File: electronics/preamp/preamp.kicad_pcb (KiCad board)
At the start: 2 copper layers, 24.8 x 24.8 mm, 33 parts, among them J1 Conn_01x01, J2 Conn_01x01, J3 Conn_01x01, J4 Conn_01x01, J5 Conn_01x01, J6 Conn_01x01, J7 Conn_01x01, Q1 BSS138L, U1 TL062, U2 TL062

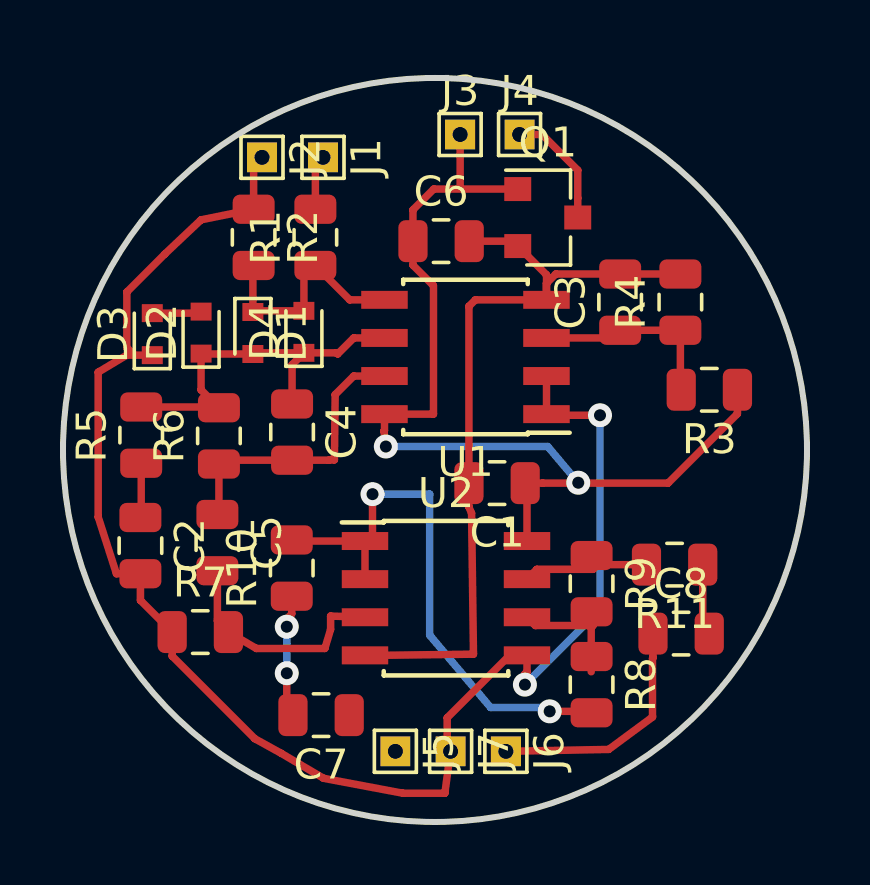
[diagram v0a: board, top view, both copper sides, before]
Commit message: Ready to make first proto
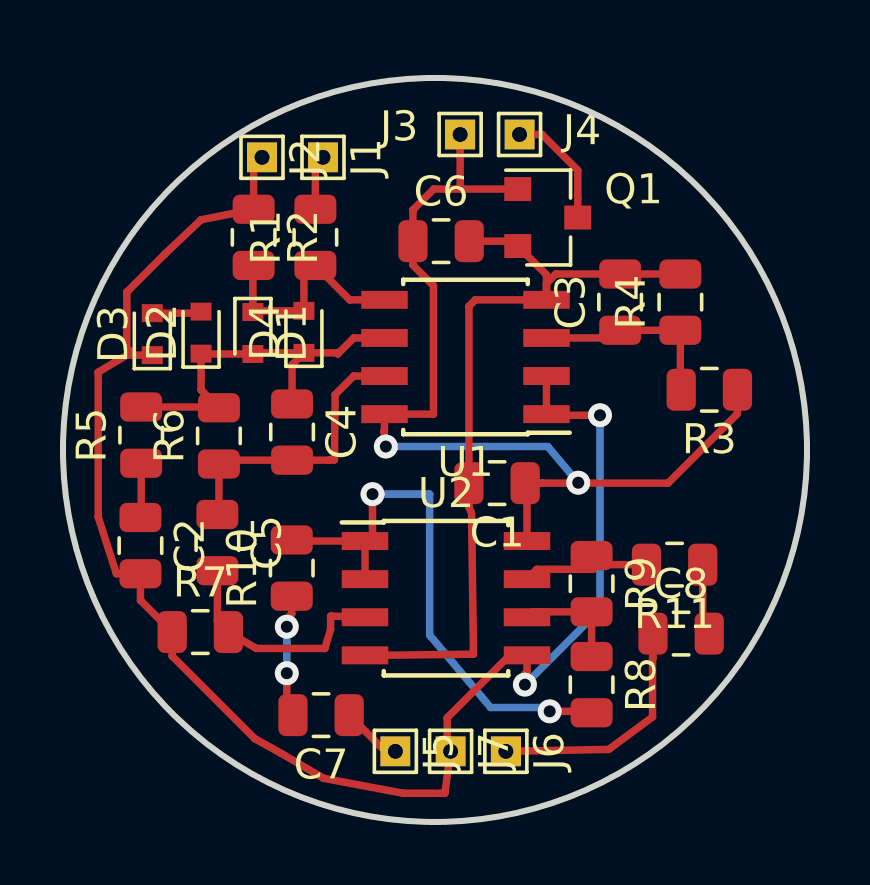
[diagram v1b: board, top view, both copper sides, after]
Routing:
- net /OUT+: track 0.00 -> 2.04 mm
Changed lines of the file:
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@@
     (thickness 1.6)
     (drawings 4)
-    (tracks 165)
+    (tracks 166)
     (zones 0)
     (modules 33)
@@
     (tags SOT-23)
     (attr smd)
-    (fp_text reference Q1 (at 0 -2.5) (layer F.SilkS)
+    (fp_text reference Q1 (at 2.8575 -0.9398) (layer F.SilkS)
       (effects (font (size 1 1) (thickness 0.15)))
     )
@@
     (pad 1 smd roundrect (at -0.9375 0 90) (size 0.975 1.4) (layers F.Cu F.Paste F.Mask) (roundrect_rratio 0.25)
       (net 17 /PRE+))
-    (model ${KISYS3DMOD}/Resistor_SMD.3dshapes/R_0805_2012Metric.wrl
+    (model ${KISYS3DMOD}/Resistors_SMD.3dshapes/R_0805.wrl
       (at (xyz 0 0 0))
       (scale (xyz 1 1 1))
@@
     (tags "test point THT pad rectangle square")
     (attr virtual)
-    (fp_text reference J3 (at 0 -1.448) (layer F.SilkS)
+    (fp_text reference J3 (at -2.032 -0.2667) (layer F.SilkS)
       (effects (font (size 1 1) (thickness 0.15)))
     )
@@
     (tags "test point THT pad rectangle square")
     (attr virtual)
-    (fp_text reference J4 (at 0 -1.448) (layer F.SilkS)
+    (fp_text reference J4 (at 2.0828 -0.1397) (layer F.SilkS)
       (effects (font (size 1 1) (thickness 0.15)))
     )
@@
     )
   )
-  (gr_text OUT (at 104.4448 113.665) (layer Eco1.User)
+  (gr_text OUT (at 100.9015 112.5855) (layer Eco1.User)
     (effects (font (size 1.5 1.5) (thickness 0.3)))
   )
-  (gr_text PWR (at 106.0704 87.0712) (layer Eco1.User)
+  (gr_text PWR (at 102.235 86.36) (layer Eco1.User)
     (effects (font (size 1.5 1.5) (thickness 0.3)))
   )
-  (gr_text IN (at 90.9828 87.7316) (layer Eco1.User)
+  (gr_text IN (at 94.996 87.757) (layer Eco1.User)
     (effects (font (size 1.5 1.5) (thickness 0.3)))
   )
@@
   (segment (start 97.666657 105.575618) (end 96.52 105.537) (width 0.25) (layer F.Cu) (net 7))
   (segment (start 96.52 105.537) (end 96.52 105.9815) (width 0.25) (layer F.Cu) (net 7))
+  (segment (start 98.3465 110.0455) (end 97.14 108.839) (width 0.25) (layer F.Cu) (net 8))
+  (segment (start 98.679 110.0455) (end 98.3465 110.0455) (width 0.25) (layer F.Cu) (net 8))
   (segment (start 95.2246 105.4618) (end 95.0595 105.6269) (width 0.25) (layer F.Cu) (net 9))
   (segment (start 95.2246 104.8743) (end 95.2246 105.4618) (width 0.25) (layer F.Cu) (net 9))
@@
   (segment (start 104.759 91.6028) (end 104.759 92.2528) (width 0.25) (layer F.Cu) (net 14))
   (segment (start 102.8192 89.4842) (end 103.5692 89.4842) (width 0.25) (layer F.Cu) (net 14))
-  (segment (start 103.343757 105.852718) (end 103.066657 105.575618) (width 0.25) (layer F.Cu) (net 15))
-  (segment (start 105.268857 105.852718) (end 103.343757 105.852718) (width 0.25) (layer F.Cu) (net 15))
-  (segment (start 105.2068 105.914775) (end 105.268857 105.852718) (width 0.25) (layer F.Cu) (net 15))
-  (segment (start 105.2068 107.3935) (end 105.2068 105.914775) (width 0.25) (layer F.Cu) (net 15))
+  (segment (start 105.2195 106.8855) (end 105.2195 105.395) (width 0.25) (layer F.Cu) (net 15))
+  (segment (start 103.247275 105.395) (end 103.066657 105.575618) (width 0.25) (layer F.Cu) (net 15))
+  (segment (start 105.2195 105.395) (end 103.247275 105.395) (width 0.25) (layer F.Cu) (net 15))
   (segment (start 97.666657 103.035618) (end 97.666657 104.305618) (width 0.25) (layer F.Cu) (net 18))
   (segment (start 95.260918 103.035618) (end 95.2246 102.9993) (width 0.25) (layer F.Cu) (net 18))
